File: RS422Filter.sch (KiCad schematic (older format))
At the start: 26 parts, among them J12 Conn_01x02, J13 Conn_01x02

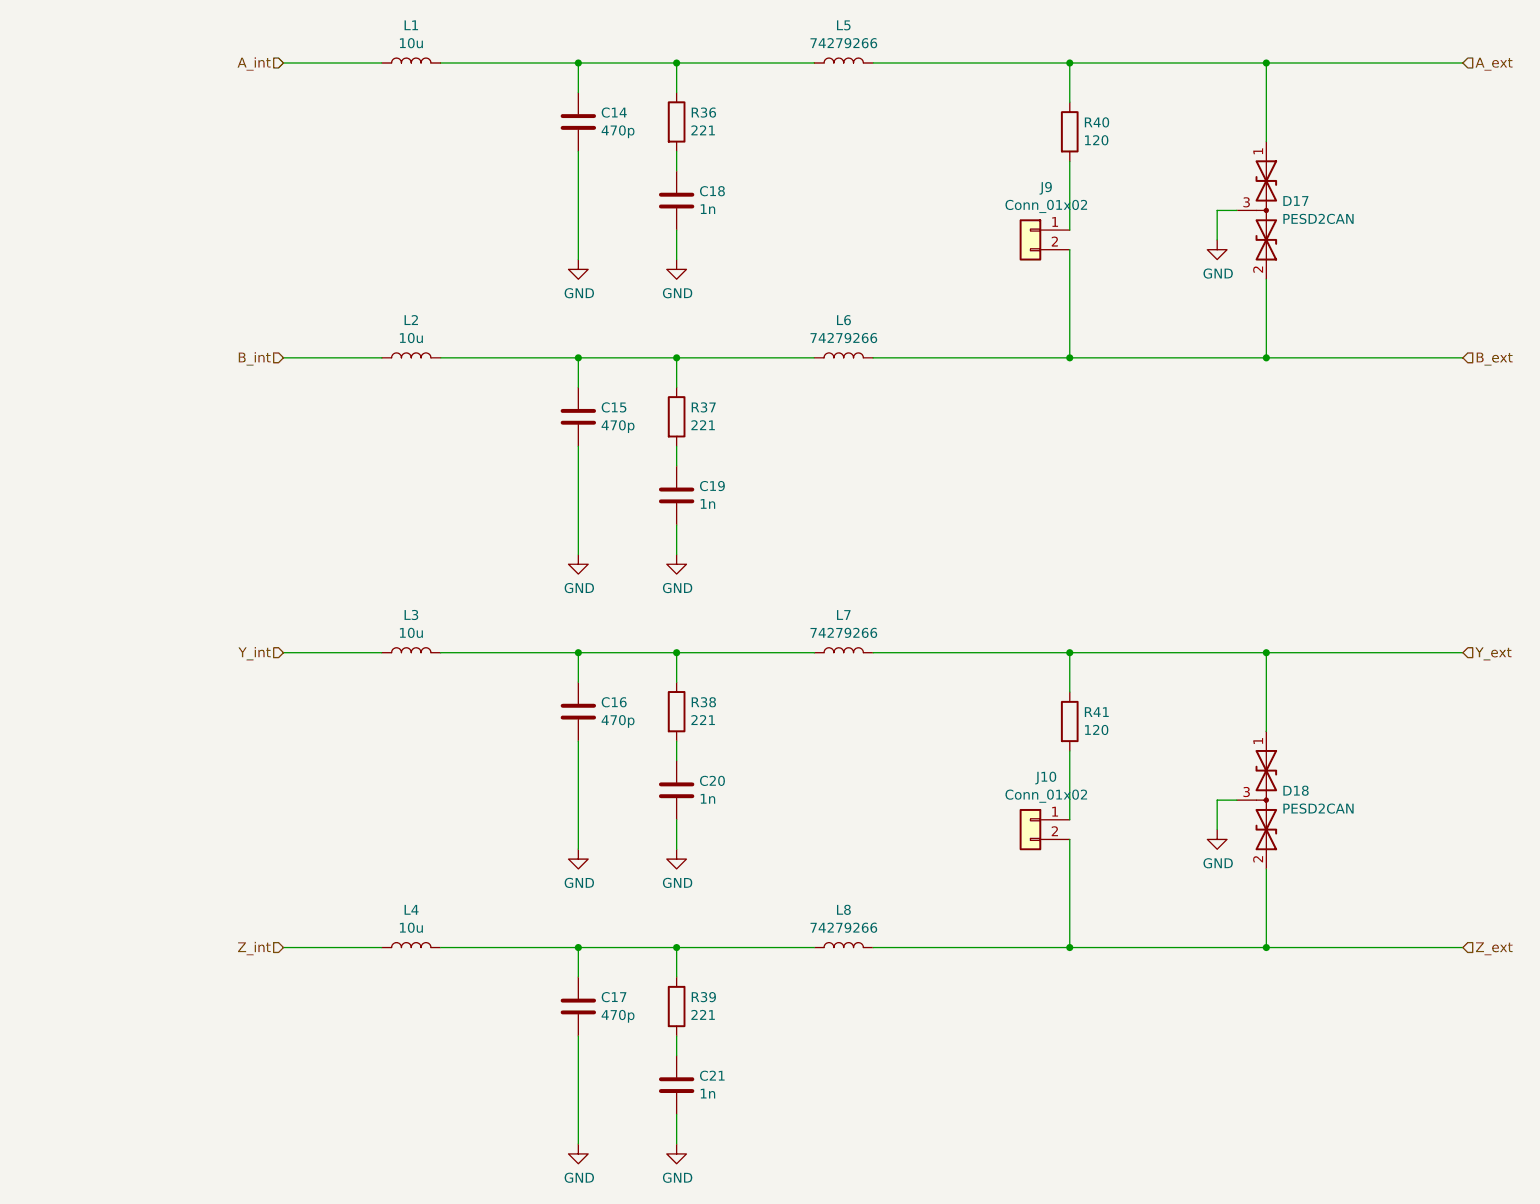
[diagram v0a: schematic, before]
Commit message: placement
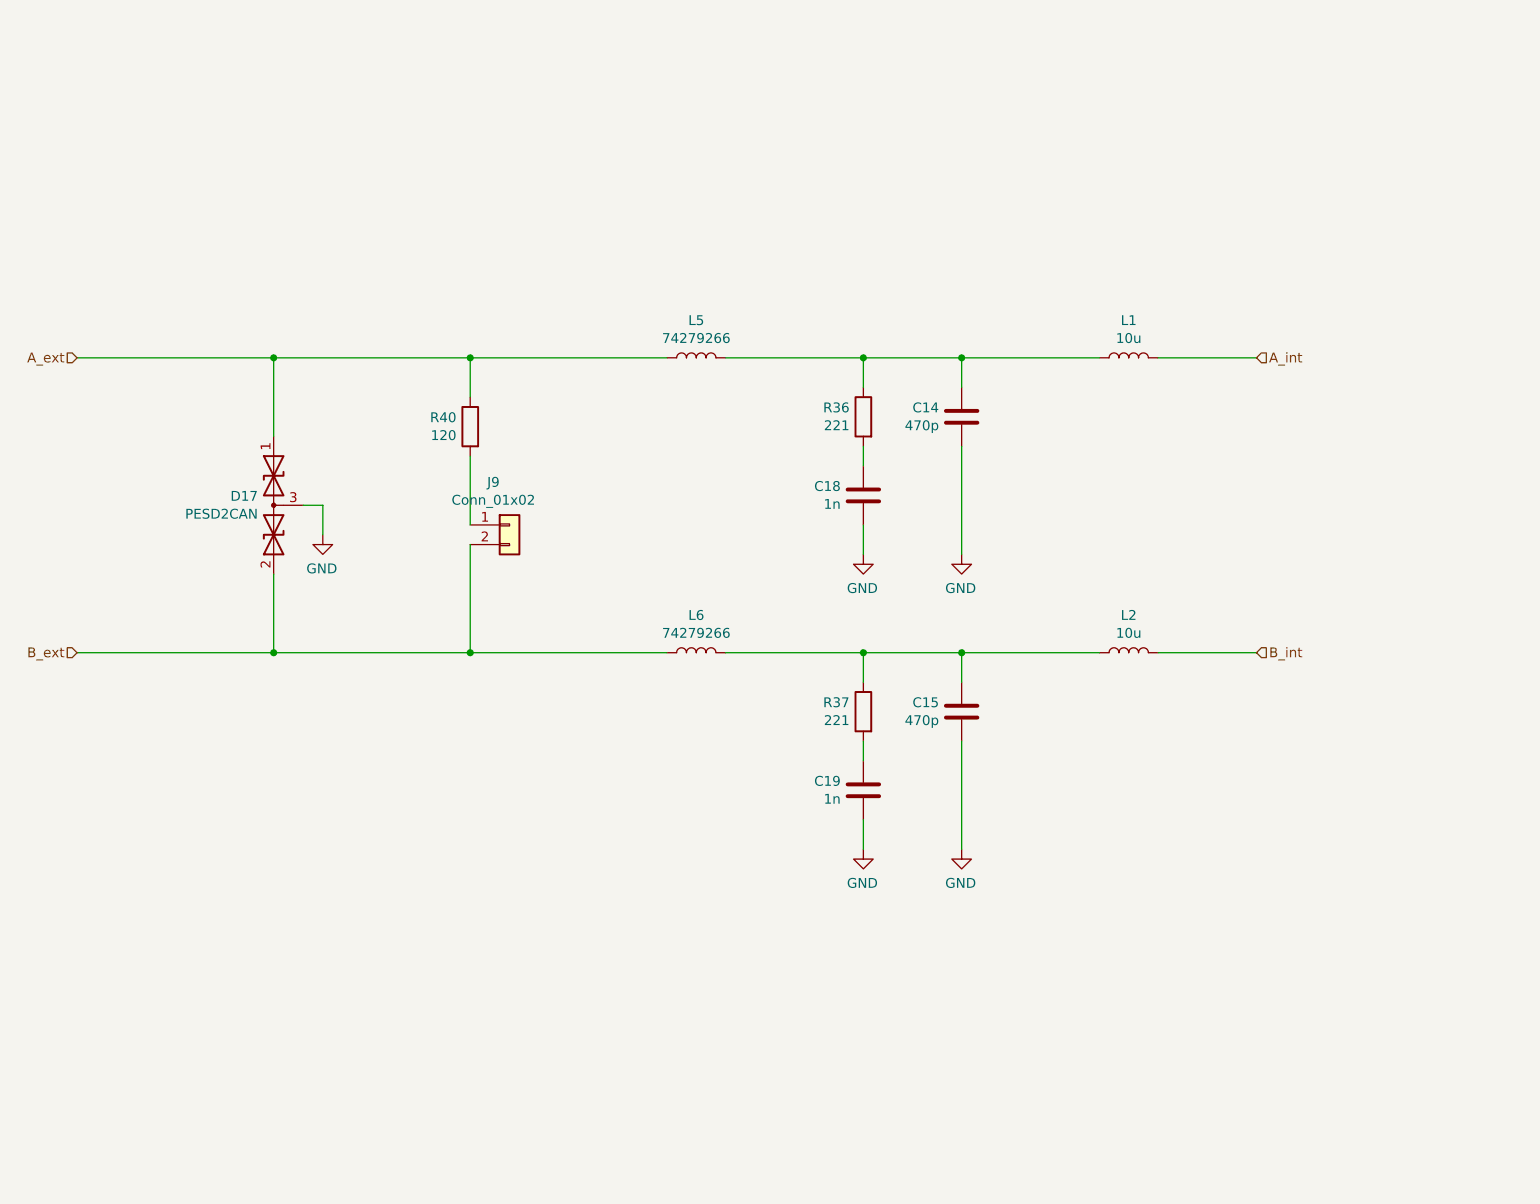
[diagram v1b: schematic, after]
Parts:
- removed C29, C30: 470p, Capacitor_SMD:C_0603_1608Metric, symbol AR2ISS:C
- removed C33, C34: 1n, Capacitor_SMD:C_0603_1608Metric, symbol AR2ISS:C
- removed D20: PESD2CAN, Package_TO_SOT_SMD:SOT-23, symbol Device:D_TVS_x2_AAC
- removed J13: Conn_01x02, symbol Connector_Generic:Conn_01x02
- removed L12, L13: 10u, symbol Device:L
- removed L16, L17: 74279266, symbol Device:L
- removed R63, R64: 221, Resistor_SMD:R_0603_1608Metric, symbol AR2ISS:R
- removed R66: 120, Resistor_SMD:R_0603_1608Metric, symbol AR2ISS:R
- D19: footprint Package_TO_SOT_SMD:SOT-23 -> Package_TO_SOT_SMD:SOT-23_Handsoldering
- J12: footprint (none) -> Connector_PinHeader_2.54mm:PinHeader_1x02_P2.54mm_Vertical
- L14, L15: footprint (none) -> Inductor_SMD:L_0603_1608Metric
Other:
- moved on the sheet: C14, C15, C18, C19, D17, J9, L1, L2, L5, L6, R36, R37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
